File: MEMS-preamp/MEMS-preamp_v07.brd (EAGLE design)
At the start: 50 x 30.1 mm, 45 parts, among them IC1 DMN2400, IC2 BQ21040, IC3 BQ297X, IC4 SC4503, IC5 TPS7A49, IC6 OPA2134, J2 Battery, SW1 SPDT

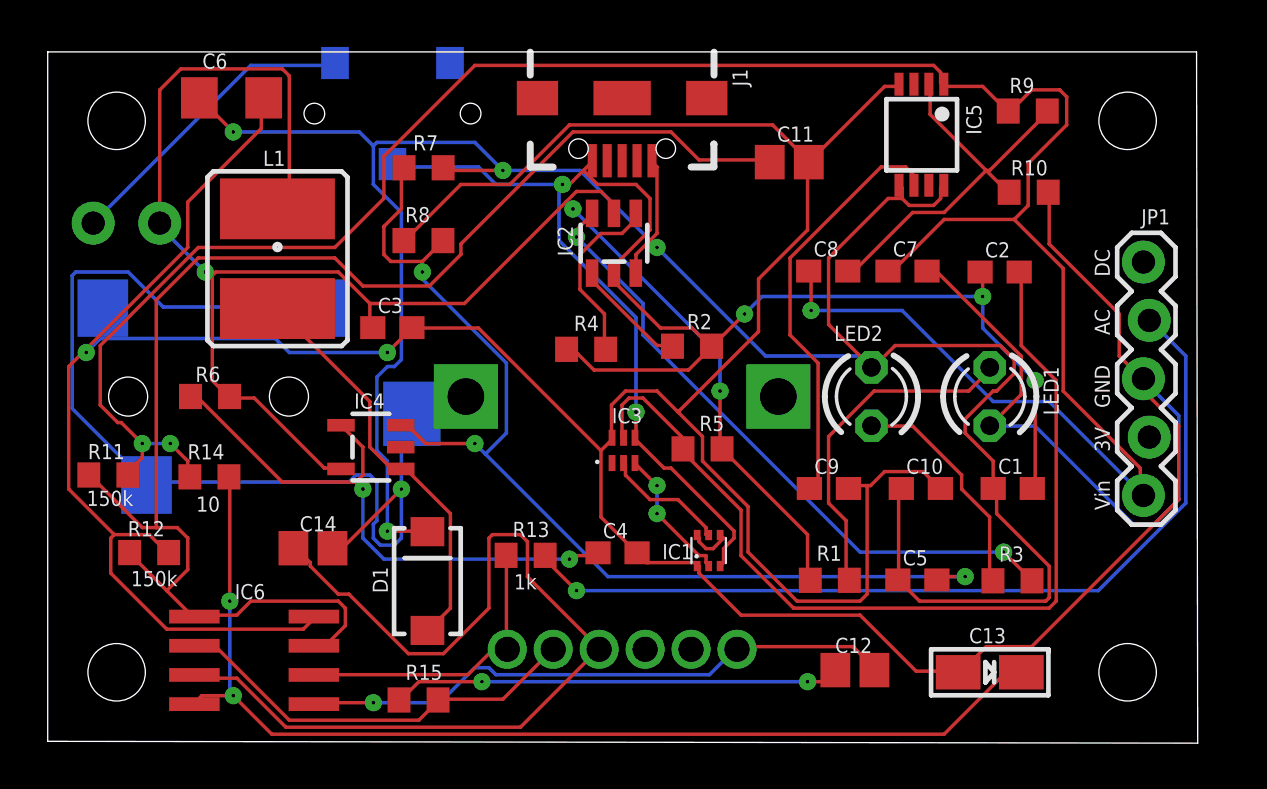
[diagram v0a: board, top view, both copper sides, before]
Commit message: upates
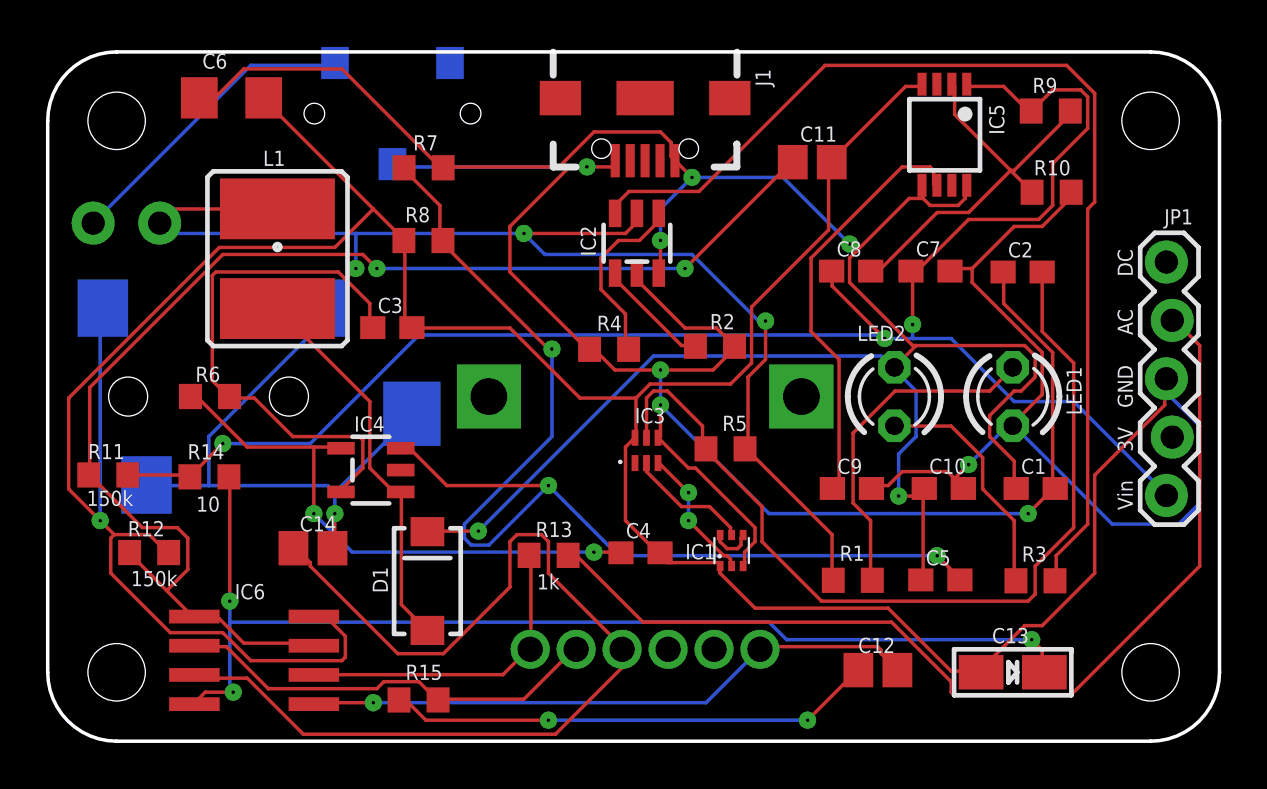
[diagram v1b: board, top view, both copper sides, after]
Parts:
- moved C1 1.00 mm to (43.0, 11.0)
- moved C10 1.00 mm to (39.0, 11.0)
- moved C11 1.00 mm to (33.3, 25.2)
- moved C12 1.00 mm to (36.1, 3.10)
- moved C13 1.00 mm to (42.0, 3.00)
- moved C2 1.00 mm to (42.4, 20.4)
- moved C4 1.00 mm to (25.8, 8.20)
- moved C5 1.00 mm to (38.9, 7.02)
- moved C7 1.00 mm to (38.4, 20.5)
- moved C8 1.00 mm to (35.0, 20.5)
- moved C9 1.00 mm to (35.0, 11.0)
- moved IC1 1.00 mm to (29.8, 8.30)
- moved IC2 1.00 mm to (25.6, 21.7)
- moved IC3 1.00 mm to (26.1, 12.7)
- moved IC4 1.00 mm to (14.1, 11.8)
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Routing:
- net GND: track 208.1 -> 177.9 mm
- net +12V: track 106.3 -> 76.5 mm
- net N$7: track 45.8 -> 25.3 mm
- net N$15: track 28.1 -> 46.2 mm, vias 2 -> 0
- net N$8: track 63.1 -> 56.9 mm, vias 0 -> 2
- net N$14: track 46.2 -> 52.1 mm
- net V+: track 106.4 -> 100.8 mm, vias 4 -> 5
- net N$3: track 38.9 -> 43.9 mm, vias 1 -> 0
- net VBAT: track 75.9 -> 78.0 mm
- net N$10: track 42.2 -> 44.3 mm
- net N$4: track 19.5 -> 21.3 mm
- net GND2: track 73.1 -> 74.8 mm, vias 5 -> 4
- net N$18: track 40.9 -> 39.4 mm
- net N$5: track 13.0 -> 14.0 mm
- net N$12: track 17.9 -> 16.9 mm
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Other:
- board size 50 x 30.1 mm -> 51 x 30 mm
